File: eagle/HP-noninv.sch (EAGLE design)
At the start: 22 parts, among them IC1 OPA2134, IC2 TLE2426CLP

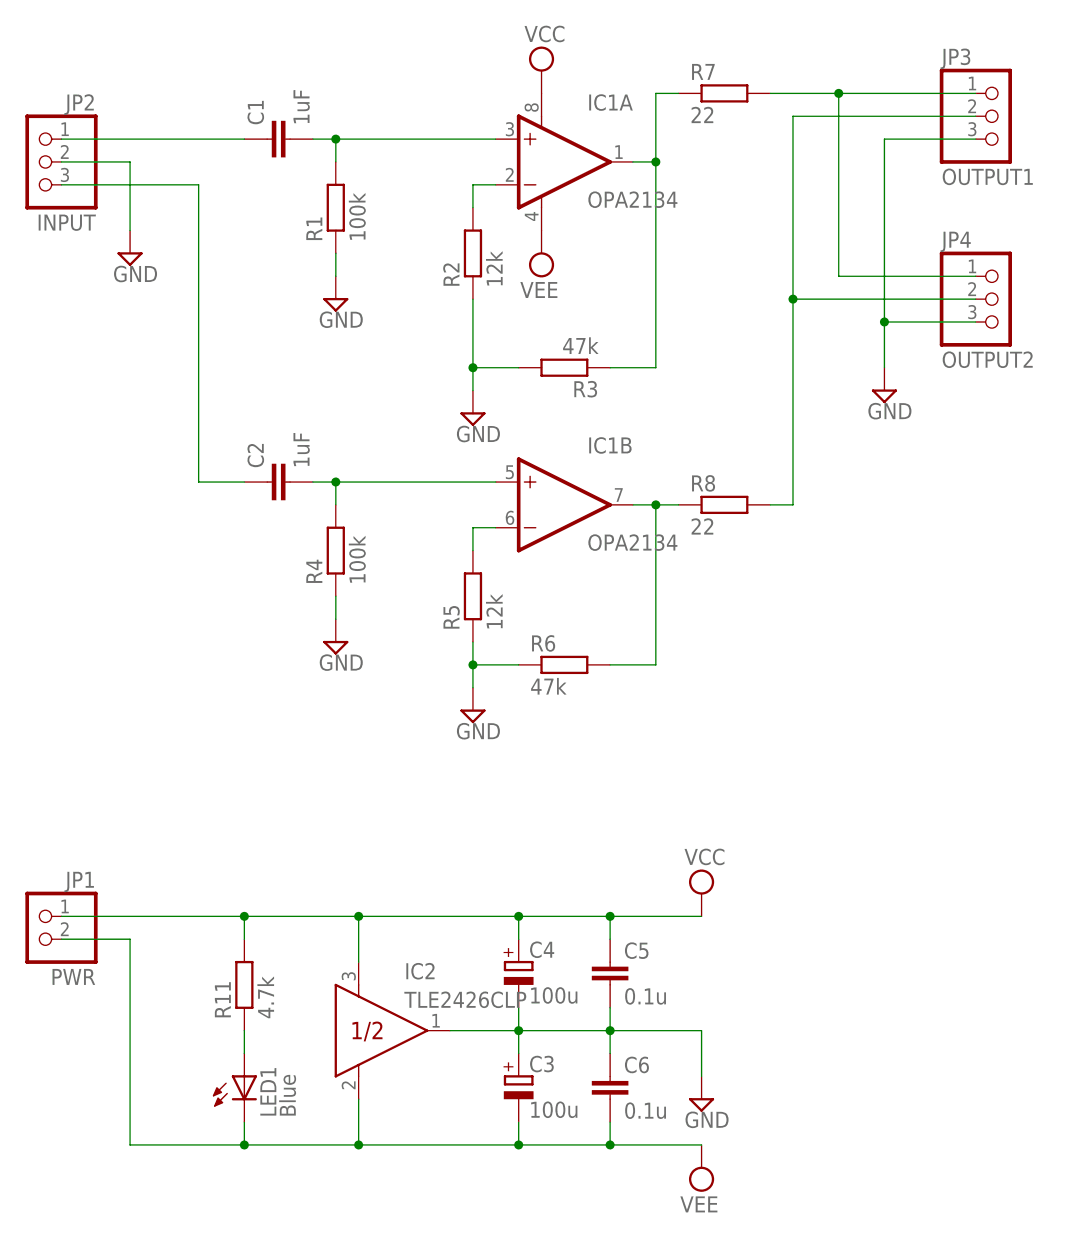
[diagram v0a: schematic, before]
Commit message: Hardware完成
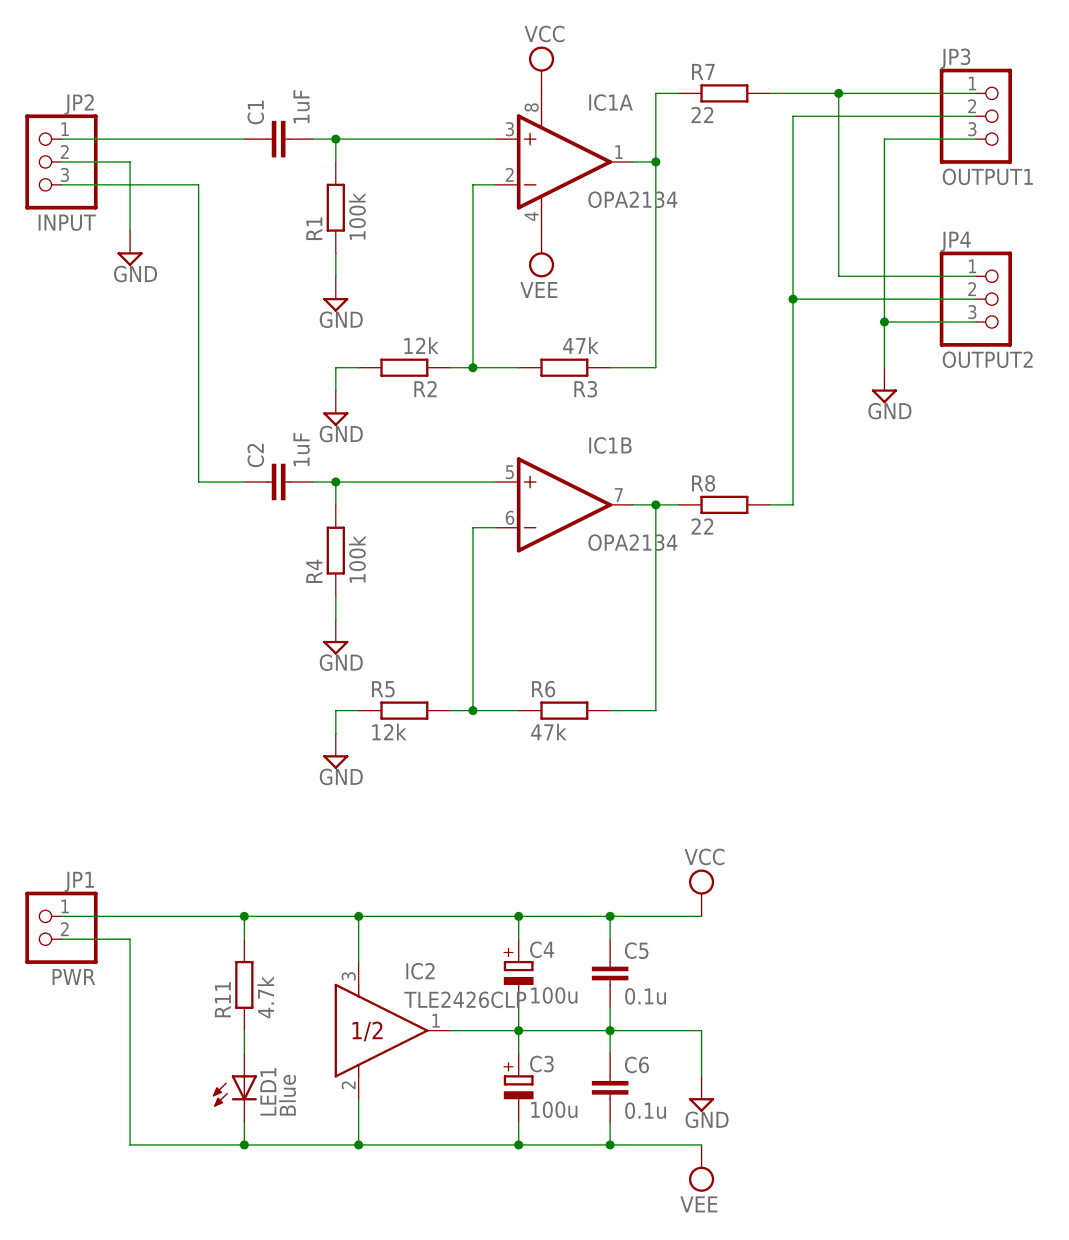
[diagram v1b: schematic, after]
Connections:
- net GND: now also R2.2; no longer R2.1, R3.2, R6.1
- net N$7: now also R2.1, R3.2; no longer R2.2
- net N$9: now also R6.1
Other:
- moved on the sheet: R2, R5, R6
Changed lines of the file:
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@@
 <instance part="IC1" gate="A" x="101.6" y="152.4"/>
 <instance part="IC1" gate="B" x="101.6" y="114.3"/>
-<instance part="R2" gate="G$1" x="91.44" y="142.24" rot="R90"/>
+<instance part="R2" gate="G$1" x="83.82" y="129.54" rot="R180"/>
 <instance part="R3" gate="G$1" x="101.6" y="129.54" rot="R180"/>
-<instance part="SUPPLY6" gate="GND" x="91.44" y="124.46"/>
+<instance part="SUPPLY6" gate="GND" x="76.2" y="124.46"/>
 <instance part="SUPPLY7" gate="G$1" x="99.06" y="162.56"/>
 <instance part="SUPPLY8" gate="G$1" x="99.06" y="142.24" rot="R180"/>
 <instance part="SUPPLY9" gate="GND" x="137.16" y="127"/>
-<instance part="R5" gate="G$1" x="91.44" y="104.14" rot="R90"/>
-<instance part="R6" gate="G$1" x="101.6" y="96.52"/>
-<instance part="SUPPLY10" gate="GND" x="91.44" y="91.44"/>
+<instance part="R5" gate="G$1" x="83.82" y="91.44"/>
+<instance part="R6" gate="G$1" x="101.6" y="91.44"/>
+<instance part="SUPPLY10" gate="GND" x="76.2" y="86.36"/>
 <instance part="JP1" gate="G$1" x="43.18" y="66.04" rot="MR0"/>
 <instance part="R11" gate="G$1" x="66.04" y="60.96" rot="R90"/>
@@
 </segment>
 <segment>
-<pinref part="R3" gate="G$1" pin="2"/>
-<wire x1="96.52" y1="129.54" x2="91.44" y2="129.54" width="0.1524" layer="91"/>
-<pinref part="R2" gate="G$1" pin="1"/>
-<wire x1="91.44" y1="129.54" x2="91.44" y2="137.16" width="0.1524" layer="91"/>
-<pinref part="SUPPLY6" gate="GND" pin="GND"/>
-<wire x1="91.44" y1="127" x2="91.44" y2="129.54" width="0.1524" layer="91"/>
-<junction x="91.44" y="129.54"/>
-</segment>
-<segment>
 <pinref part="SUPPLY5" gate="GND" pin="GND"/>
 <pinref part="R4" gate="G$1" pin="1"/>
 <wire x1="76.2" y1="101.6" x2="76.2" y2="104.14" width="0.1524" layer="91"/>
-</segment>
-<segment>
-<pinref part="R5" gate="G$1" pin="1"/>
-<wire x1="91.44" y1="99.06" x2="91.44" y2="96.52" width="0.1524" layer="91"/>
-<pinref part="SUPPLY10" gate="GND" pin="GND"/>
-<pinref part="R6" gate="G$1" pin="1"/>
-<wire x1="91.44" y1="96.52" x2="91.44" y2="93.98" width="0.1524" layer="91"/>
-<wire x1="96.52" y1="96.52" x2="91.44" y2="96.52" width="0.1524" layer="91"/>
-<junction x="91.44" y="96.52"/>
 </segment>
 <segment>
@@
 <wire x1="53.34" y1="152.4" x2="53.34" y2="144.78" width="0.1524" layer="91"/>
 </segment>
+<segment>
+<pinref part="R2" gate="G$1" pin="2"/>
+<pinref part="SUPPLY6" gate="GND" pin="GND"/>
+<wire x1="78.74" y1="129.54" x2="76.2" y2="129.54" width="0.1524" layer="91"/>
+<wire x1="76.2" y1="129.54" x2="76.2" y2="127" width="0.1524" layer="91"/>
+</segment>
+<segment>
+<pinref part="SUPPLY10" gate="GND" pin="GND"/>
+<wire x1="76.2" y1="91.44" x2="76.2" y2="88.9" width="0.1524" layer="91"/>
+<pinref part="R5" gate="G$1" pin="1"/>
+<wire x1="76.2" y1="91.44" x2="78.74" y2="91.44" width="0.1524" layer="91"/>
+</segment>
 </net>
 <net name="N$5" class="0">
@@
 <net name="N$7" class="0">
 <segment>
-<pinref part="R2" gate="G$1" pin="2"/>
-<wire x1="91.44" y1="147.32" x2="91.44" y2="149.86" width="0.1524" layer="91"/>
 <pinref part="IC1" gate="A" pin="-IN"/>
 <wire x1="91.44" y1="149.86" x2="93.98" y2="149.86" width="0.1524" layer="91"/>
+<pinref part="R2" gate="G$1" pin="1"/>
+<pinref part="R3" gate="G$1" pin="2"/>
+<wire x1="88.9" y1="129.54" x2="91.44" y2="129.54" width="0.1524" layer="91"/>
+<wire x1="91.44" y1="129.54" x2="96.52" y2="129.54" width="0.1524" layer="91"/>
+<wire x1="91.44" y1="149.86" x2="91.44" y2="129.54" width="0.1524" layer="91"/>
+<junction x="91.44" y="129.54"/>
 </segment>
 </net>
@@
 <net name="N$9" class="0">
 <segment>
-<pinref part="R5" gate="G$1" pin="2"/>
-<wire x1="91.44" y1="109.22" x2="91.44" y2="111.76" width="0.1524" layer="91"/>
 <pinref part="IC1" gate="B" pin="-IN"/>
 <wire x1="91.44" y1="111.76" x2="93.98" y2="111.76" width="0.1524" layer="91"/>
+<pinref part="R6" gate="G$1" pin="1"/>
+<wire x1="91.44" y1="91.44" x2="96.52" y2="91.44" width="0.1524" layer="91"/>
+<wire x1="91.44" y1="111.76" x2="91.44" y2="91.44" width="0.1524" layer="91"/>
+<pinref part="R5" gate="G$1" pin="2"/>
+<wire x1="88.9" y1="91.44" x2="91.44" y2="91.44" width="0.1524" layer="91"/>
+<junction x="91.44" y="91.44"/>
 </segment>
 </net>
@@
 <segment>
 <pinref part="IC1" gate="B" pin="OUT"/>
-<wire x1="109.22" y1="114.3" x2="111.76" y2="114.3" width="0.1524" layer="91"/>
-<wire x1="111.76" y1="114.3" x2="111.76" y2="96.52" width="0.1524" layer="91"/>
-<pinref part="R6" gate="G$1" pin="2"/>
-<wire x1="106.68" y1="96.52" x2="111.76" y2="96.52" width="0.1524" layer="91"/>
 <pinref part="R8" gate="G$1" pin="1"/>
 <wire x1="114.3" y1="114.3" x2="111.76" y2="114.3" width="0.1524" layer="91"/>
+<pinref part="R6" gate="G$1" pin="2"/>
+<wire x1="111.76" y1="114.3" x2="109.22" y2="114.3" width="0.1524" layer="91"/>
+<wire x1="106.68" y1="91.44" x2="111.76" y2="91.44" width="0.1524" layer="91"/>
+<wire x1="111.76" y1="91.44" x2="111.76" y2="114.3" width="0.1524" layer="91"/>
 <junction x="111.76" y="114.3"/>
 </segment>
